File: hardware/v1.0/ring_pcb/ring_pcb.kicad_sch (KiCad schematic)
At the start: 13 parts

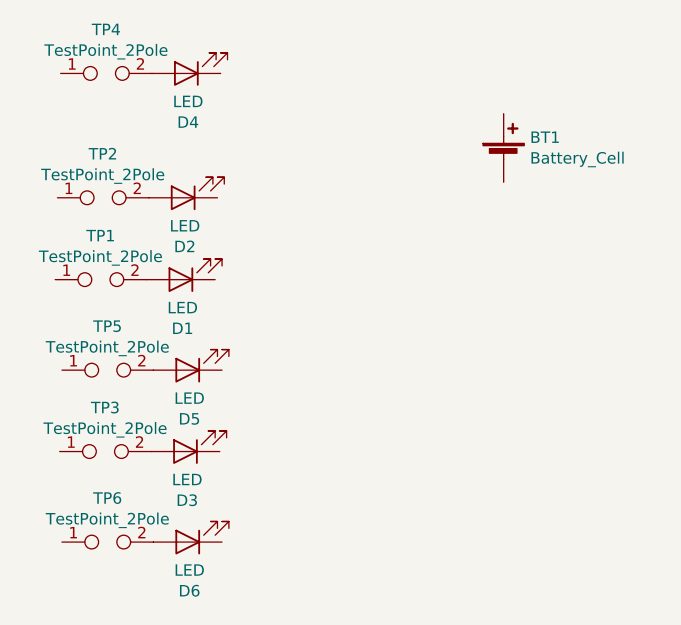
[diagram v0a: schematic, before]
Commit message: First v0.1 cut
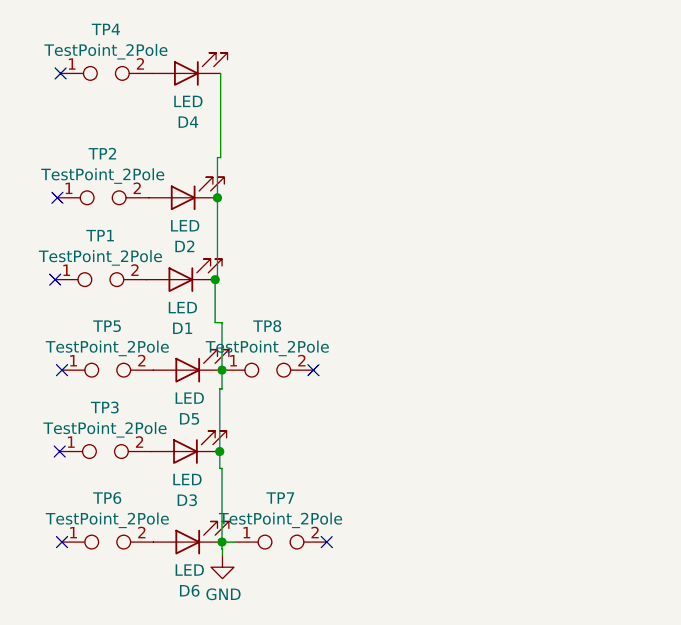
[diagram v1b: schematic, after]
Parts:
- removed BT1: Battery_Cell, Battery:BatteryHolder_LINX_BAT-HLD-012-SMT, symbol Device:Battery_Cell
- added TP7, TP8: TestPoint_2Pole, Connector_Wire:SolderWirePad_1x02_P3.81mm_Drill1.2mm, symbol Connector:TestPoint_2Pole
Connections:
- net GND: now reaches D4.1 (K)
- net GND: now also D1.1 (K), D2.1 (K), D3.1 (K), D5.1 (K), D6.1 (K), TP7.1, TP8.1
- no-connect marks 0 -> 8
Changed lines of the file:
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@@
 (kicad_sch (version 20201015) (generator eeschema)
   (paper "A4")
+  (junction (at 125.6284 87.7824) (diameter 1.016) (color 0 0 0 0))
+  (junction (at 125.8824 78.6892) (diameter 1.016) (color 0 0 0 0))
+  (junction (at 126.1364 106.8832) (diameter 1.016) (color 0 0 0 0))
+  (junction (at 126.3904 97.8408) (diameter 1.016) (color 0 0 0 0))
+  (junction (at 126.3904 116.9416) (diameter 1.016) (color 0 0 0 0))
+  (no_connect (at 108.458 64.8716))
+  (no_connect (at 107.8484 87.7824))
+  (no_connect (at 108.1024 78.6892))
+  (no_connect (at 108.3564 106.8832))
+  (no_connect (at 108.6104 97.8408))
+  (no_connect (at 108.6104 116.9416))
+  (no_connect (at 138.0236 116.9416))
+  (no_connect (at 136.5504 97.8408))
+  (wire (pts (xy 125.6284 87.7824) (xy 125.6284 92.5576))
+    (stroke (width 0) (type solid) (color 0 0 0 0))
+  )
+  (wire (pts (xy 125.6284 87.7824) (xy 125.8824 87.7824))
+    (stroke (width 0) (type solid) (color 0 0 0 0))
+  )
+  (wire (pts (xy 125.6284 92.5576) (xy 126.3904 92.5576))
+    (stroke (width 0) (type solid) (color 0 0 0 0))
+  )
+  (wire (pts (xy 125.8824 74.2188) (xy 125.8824 78.6892))
+    (stroke (width 0) (type solid) (color 0 0 0 0))
+  )
+  (wire (pts (xy 125.8824 78.6892) (xy 125.8824 87.7824))
+    (stroke (width 0) (type solid) (color 0 0 0 0))
+  )
+  (wire (pts (xy 126.1364 99.9236) (xy 126.3904 99.9236))
+    (stroke (width 0) (type solid) (color 0 0 0 0))
+  )
+  (wire (pts (xy 126.1364 106.8832) (xy 126.1364 99.9236))
+    (stroke (width 0) (type solid) (color 0 0 0 0))
+  )
+  (wire (pts (xy 126.1364 108.7628) (xy 126.1364 106.8832))
+    (stroke (width 0) (type solid) (color 0 0 0 0))
+  )
+  (wire (pts (xy 126.238 64.8716) (xy 126.238 74.2188))
+    (stroke (width 0) (type solid) (color 0 0 0 0))
+  )
+  (wire (pts (xy 126.238 74.2188) (xy 125.8824 74.2188))
+    (stroke (width 0) (type solid) (color 0 0 0 0))
+  )
+  (wire (pts (xy 126.3904 92.5576) (xy 126.3904 97.8408))
+    (stroke (width 0) (type solid) (color 0 0 0 0))
+  )
+  (wire (pts (xy 126.3904 99.9236) (xy 126.3904 97.8408))
+    (stroke (width 0) (type solid) (color 0 0 0 0))
+  )
+  (wire (pts (xy 126.3904 108.7628) (xy 126.1364 108.7628))
+    (stroke (width 0) (type solid) (color 0 0 0 0))
+  )
+  (wire (pts (xy 126.3904 108.7628) (xy 126.3904 116.9416))
+    (stroke (width 0) (type solid) (color 0 0 0 0))
+  )
+  (wire (pts (xy 126.3904 116.9416) (xy 126.3904 117.7036))
+    (stroke (width 0) (type solid) (color 0 0 0 0))
+  )
+  (wire (pts (xy 126.3904 116.9416) (xy 127.8636 116.9416))
+    (stroke (width 0) (type solid) (color 0 0 0 0))
+  )
+  (wire (pts (xy 126.3904 117.7036) (xy 126.4412 117.7036))
+    (stroke (width 0) (type solid) (color 0 0 0 0))
+  )
+  (wire (pts (xy 126.4412 117.7036) (xy 126.4412 118.4656))
+    (stroke (width 0) (type solid) (color 0 0 0 0))
+  )
+  (symbol (lib_id "power:GND") (at 126.4412 118.4656 0) (unit 1)
+    (in_bom yes) (on_board yes)
+    (property "Reference" "#PWR0101" (id 0) (at 126.4412 124.8156 0)
+      (effects (font (size 1.27 1.27)) hide)
+    )
+    (property "Value" "GND" (id 1) (at 126.5555 122.79 0))
+    (property "Footprint" "" (id 2) (at 126.4412 118.4656 0)
+      (effects (font (size 1.27 1.27)) hide)
+    )
+    (property "Datasheet" "" (id 3) (at 126.4412 118.4656 0)
+      (effects (font (size 1.27 1.27)) hide)
+    )
+  )
   (symbol (lib_id "Connector:TestPoint_2Pole") (at 112.9284 87.7824 0) (unit 1)
     (in_bom yes) (on_board yes)
@@
     )
   )
+  (symbol (lib_id "Connector:TestPoint_2Pole") (at 131.4704 97.8408 0) (unit 1)
+    (in_bom yes) (on_board yes)
+    (property "Reference" "TP8" (id 0) (at 131.4704 92.9956 0))
+    (property "Value" "TestPoint_2Pole" (id 1) (at 131.4704 95.2943 0))
+    (property "Footprint" "Connector_Wire:SolderWirePad_1x02_P3.81mm_Drill1.2mm" (id 2) (at 131.4704 97.8408 0)
+      (effects (font (size 1.27 1.27)) hide)
+    )
+    (property "Datasheet" "~" (id 3) (at 131.4704 97.8408 0)
+      (effects (font (size 1.27 1.27)) hide)
+    )
+  )
+  (symbol (lib_id "Connector:TestPoint_2Pole") (at 132.9436 116.9416 0) (unit 1)
+    (in_bom yes) (on_board yes)
+    (property "Reference" "TP7" (id 0) (at 132.9436 112.0964 0))
+    (property "Value" "TestPoint_2Pole" (id 1) (at 132.9436 114.3951 0))
+    (property "Footprint" "Connector_Wire:SolderWirePad_1x02_P3.81mm_Drill1.2mm" (id 2) (at 132.9436 116.9416 0)
+      (effects (font (size 1.27 1.27)) hide)
+    )
+    (property "Datasheet" "~" (id 3) (at 132.9436 116.9416 0)
+      (effects (font (size 1.27 1.27)) hide)
+    )
+  )
   (symbol (lib_id "Device:LED") (at 121.8184 87.7824 180) (unit 1)
     (in_bom yes) (on_board yes)
@@
     )
   )
-  (symbol (lib_id "Device:Battery_Cell") (at 157.6832 74.422 0) (unit 1)
-    (in_bom yes) (on_board yes)
-    (property "Reference" "BT1" (id 0) (at 160.6043 72.0026 0)
-      (effects (font (size 1.27 1.27)) (justify left))
-    )
-    (property "Value" "Battery_Cell" (id 1) (at 160.6043 74.3013 0)
-      (effects (font (size 1.27 1.27)) (justify left))
-    )
-    (property "Footprint" "Battery:BatteryHolder_LINX_BAT-HLD-012-SMT" (id 2) (at 157.6832 72.898 90)
-      (effects (font (size 1.27 1.27)) hide)
-    )
-    (property "Datasheet" "~" (id 3) (at 157.6832 72.898 90)
-      (effects (font (size 1.27 1.27)) hide)
-    )
-  )
   (sheet_instances
     (path "/" (page "1"))
   )
   (symbol_instances
-    (path "/7f23df0d-c5f1-4fc3-b7fe-c7e90ce83fc7"
-      (reference "BT1") (unit 1) (value "Battery_Cell") (footprint "Battery:BatteryHolder_LINX_BAT-HLD-012-SMT")
+    (path "/3a654da8-ff45-4a1d-a535-cda78a2ba341"
+      (reference "#PWR0101") (unit 1) (value "GND") (footprint "")
     )
     (path "/f86d50c5-128d-459b-974c-e0abf9f5794b"
@@
       (reference "TP6") (unit 1) (value "TestPoint_2Pole") (footprint "TestPoint:TestPoint_2Pads_Pitch2.54mm_Drill0.8mm")
     )
-  )
+    (path "/5d1d4b9e-26cd-49ce-9a48-1f08d40d65d5"
+      (reference "TP7") (unit 1) (value "TestPoint_2Pole") (footprint "Connector_Wire:SolderWirePad_1x02_P3.81mm_Drill1.2mm")
+    )
+    (path "/695df2d6-462a-4d24-81ce-81457d22234a"
+      (reference "TP8") (unit 1) (value "TestPoint_2Pole") (footprint "Connector_Wire:SolderWirePad_1x02_P3.81mm_Drill1.2mm")
+    )
+  )
